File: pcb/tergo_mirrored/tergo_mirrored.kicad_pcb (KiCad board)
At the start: 2 copper layers, 140.5 x 100.6 mm, 63 parts, among them J3 MJ-4PP-9, SW1 SW_PUSH, SW10 SW_PUSH, SW11 SW_PUSH, SW12 SW_PUSH, SW13 SW_PUSH, SW14 SW_PUSH, SW15 SW_PUSH, SW16 SW_PUSH, SW17 SW_PUSH, SW18 SW_PUSH, SW19 SW_RESET, SW2 SW_PUSH, SW20 SW_PUSH, SW21 SW_PUSH, SW22 SW_PUSH, SW23 SW_PUSH, SW3 SW_PUSH, SW4 SW_PUSH, SW5 SW_PUSH, SW6 SW_PUSH, SW7 SW_PUSH, SW8 SW_PUSH, SW9 SW_PUSH, U1 Raspberry_Pie_Pico

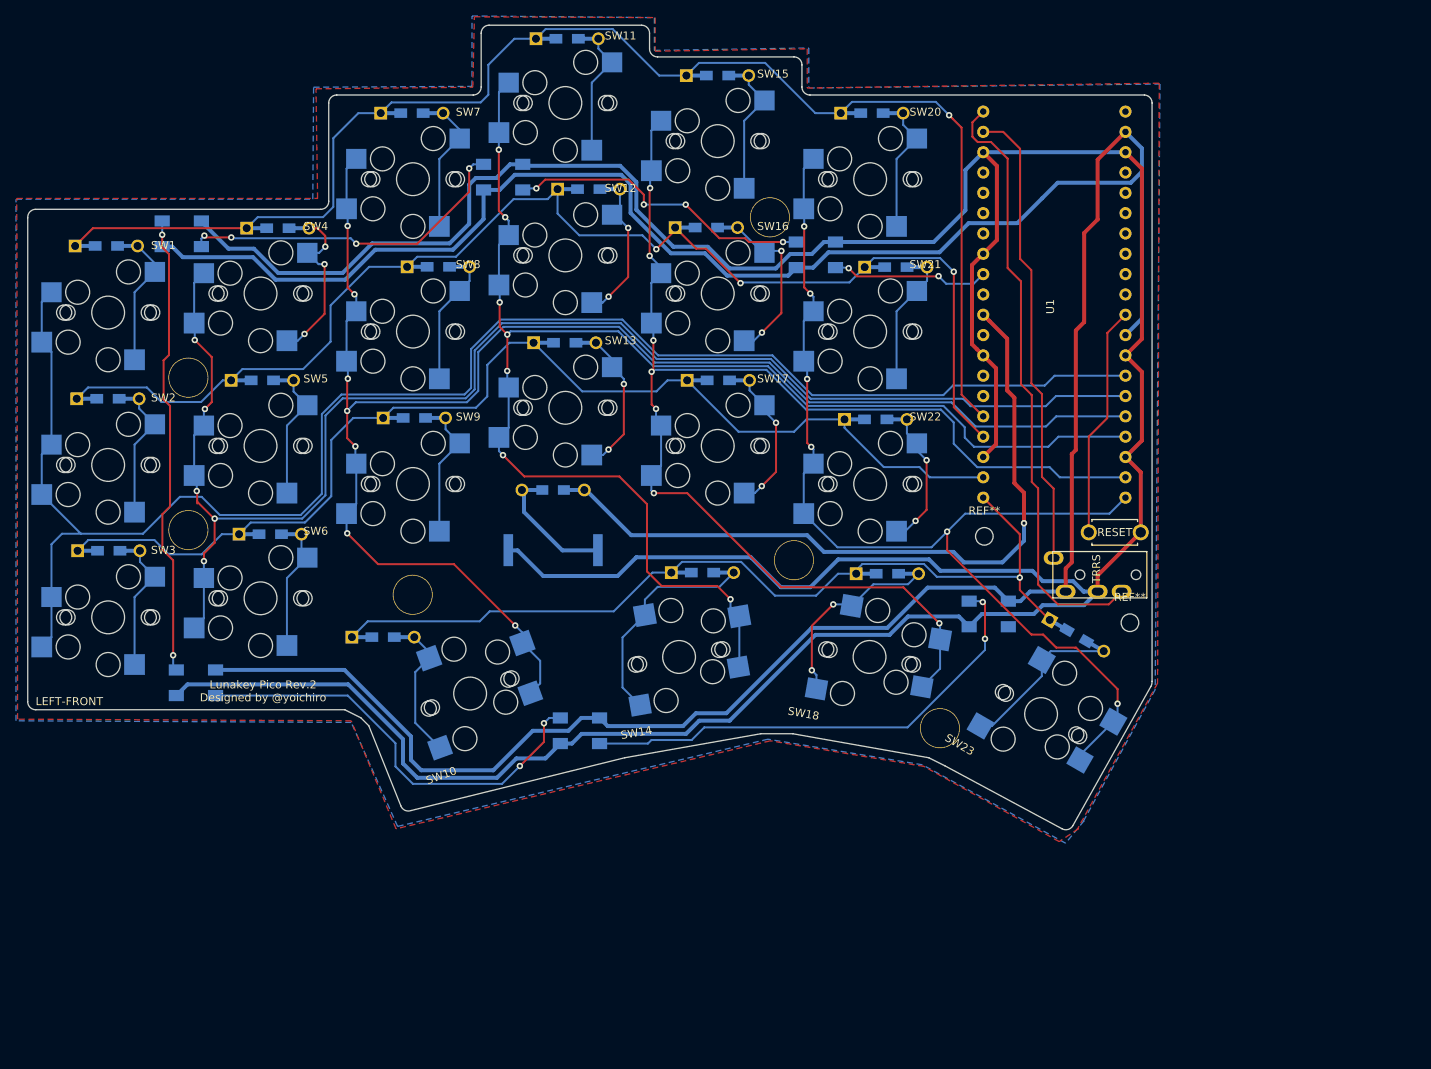
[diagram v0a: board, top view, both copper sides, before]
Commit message: wip
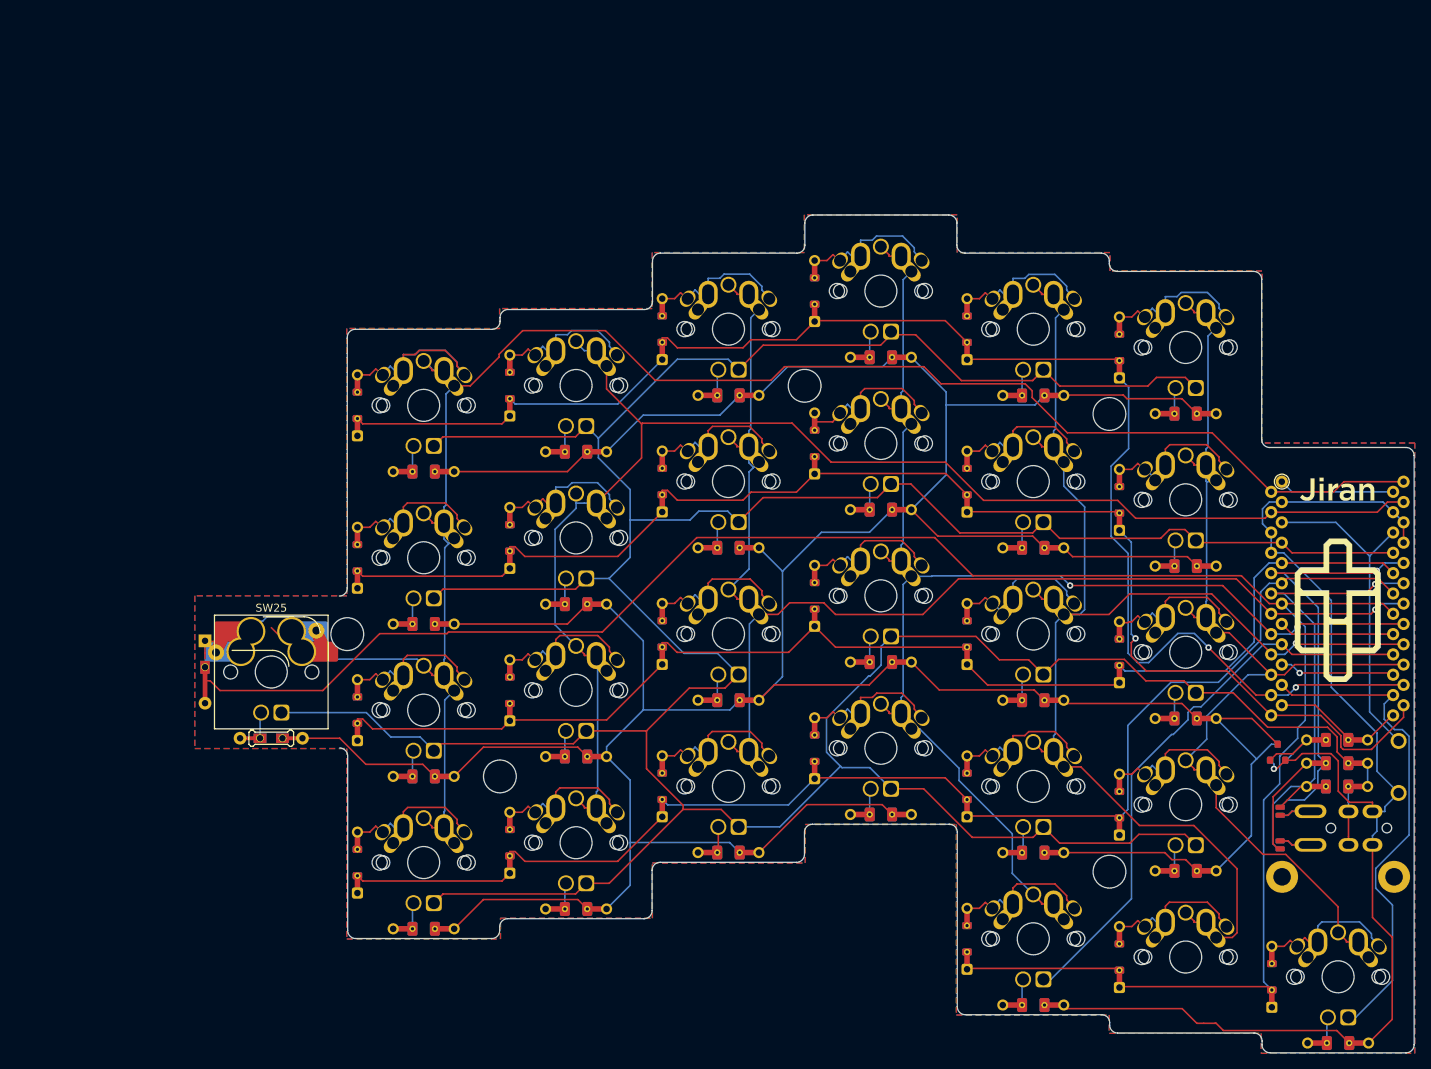
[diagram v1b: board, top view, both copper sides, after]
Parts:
- removed J3: MJ-4PP-9, kbd:MJ-4PP-9_1side
- removed LS1: PKLCS1212E4001-R1, _tergo_lib:PKLCS1212E4001-R1
- removed REF** (x2): COVER, MountingHole:MountingHole_2.2mm_M2
- removed Ref** (x6): Val**, kbd:HOLE
- added D23: 1N4148, Used_Footprints:Diode_Hybrid_SOD-123, F.Cu at (180.4, 180.7)
- added D24: 1N4148, Used_Footprints:Diode_Hybrid_SOD-123, F.Cu at (199.5, 183.0)
- added D25: 1N4148, _tergo_lib:Diode-Hybrid-2sided, F.Cu at (85.2, 166.4)
- added D26: 1N4148, Used_Footprints:Diode_Hybrid_SOD-123, F.Cu at (180.4, 199.7)
- added D27: 1N4148, Used_Footprints:Diode_Hybrid_SOD-123, F.Cu at (199.5, 202.0)
- added D28: 1N4148, Used_Footprints:Diode_Hybrid_SOD-123, F.Cu at (218.5, 204.5)
- added D29: LED_Small, Used_Footprints:LED, F.Cu at (112.5, 138.1)
- added D30: LED_Small, Used_Footprints:LED, F.Cu at (131.5, 135.6)
- added D31: LED_Small, Used_Footprints:LED, F.Cu at (150.6, 128.6)
- added D32: LED_Small, Used_Footprints:LED, F.Cu at (169.6, 123.8)
- added D33: LED_Small, Used_Footprints:LED, F.Cu at (188.7, 128.6)
- added D34: LED_Small, Used_Footprints:LED, F.Cu at (207.7, 130.9)
- added D35: LED_Small, Used_Footprints:LED, F.Cu at (112.5, 157.2)
- added D36: LED_Small, Used_Footprints:LED, F.Cu at (131.5, 154.7)
- added D37: LED_Small, Used_Footprints:LED, F.Cu at (150.6, 147.6)
- added D38: LED_Small, Used_Footprints:LED, F.Cu at (169.6, 142.9)
- added D39: LED_Small, Used_Footprints:LED, F.Cu at (188.7, 147.7)
- added D40: LED_Small, Used_Footprints:LED, F.Cu at (207.7, 149.9)
- added D41: LED_Small, Used_Footprints:LED, F.Cu at (112.5, 176.2)
- added D42: LED_Small, Used_Footprints:LED, F.Cu at (131.5, 173.7)
- added D43: LED_Small, Used_Footprints:LED, F.Cu at (150.6, 166.7)
- added D44: LED_Small, Used_Footprints:LED, F.Cu at (169.6, 161.9)
- added D50: LED_Small, Used_Footprints:LED, F.Cu at (169.6, 181.0)
- added D52: LED_Small, Used_Footprints:LED, F.Cu at (207.7, 188.0)
- added D53: LED_Small, Used_Footprints:LED, F.Cu at (93.4, 171.5)
- added D54: LED_Small, Used_Footprints:LED, F.Cu at (188.7, 204.8)
- added D56: LED_Small, Used_Footprints:LED, F.Cu at (226.8, 209.6)
- added G1: LOGO, Used_Footprints:Silk_Logo_Old, B.Cu at (226.7, 156.2)
- added G2: LOGO, Used_Footprints:Silk_Logo_Old, F.Cu at (226.8, 156.2)
- added H1: CaseHole, Used_Footprints:MountHole, F.Cu at (102.9, 161.6)
- added H2: CaseHole, Used_Footprints:MountHole, F.Cu at (122.0, 179.4)
- added H3: CaseHole, Used_Footprints:MountHole, F.Cu at (160.1, 130.6)
- added H6: CaseHole, Used_Footprints:MountHole, F.Cu at (198.2, 134.1)
- added H7: CaseHole, Used_Footprints:MountHole, F.Cu at (198.2, 191.3)
- added H8: CoverHole, Used_Footprints:CoverHole, F.Cu at (233.8, 192.0)
- added H9: CoverHole, Used_Footprints:CoverHole, F.Cu at (219.8, 192.0)
- added J1: TRRS, Used_Footprints:TRSS_DUAL_THT, F.Cu at (234.4, 185.9)
- added JP2: Jumper, 1kbd:jumper, B.Cu at (219.6, 183.8)
- added JP3: Jumper, 1kbd:jumper, F.Cu at (219.6, 183.8)
- added JP4: Jumper, 1kbd:jumper, F.Cu at (219.6, 188.0)
- added JP5: Jumper, 1kbd:jumper, B.Cu at (219.6, 188.0)
- added Q1: 2N7002, Used_Footprints:SOT-23, F.Cu at (219.2, 176.5)
- added R10: 330R, Used_Footprints:Resistor_Hybrid_1205, F.Cu at (169.6, 146.1)
- added R11: 330R, Used_Footprints:Resistor_Hybrid_1205, F.Cu at (188.7, 150.9)
- added R12: 330R, Used_Footprints:Resistor_Hybrid_1205, F.Cu at (207.7, 153.1)
- added R13: 330R, Used_Footprints:Resistor_Hybrid_1205, F.Cu at (112.5, 179.4)
- added R14: 330R, Used_Footprints:Resistor_Hybrid_1205, F.Cu at (131.5, 177.0)
- added R15: 330R, Used_Footprints:Resistor_Hybrid_1205, F.Cu at (150.6, 169.9)
- added R16: 330R, Used_Footprints:Resistor_Hybrid_1205, F.Cu at (169.6, 165.1)
- added R17: 330R, Used_Footprints:Resistor_Hybrid_1205, F.Cu at (188.7, 169.9)
- added R18: 330R, Used_Footprints:Resistor_Hybrid_1205, F.Cu at (207.7, 172.2)
- added R19: 330R, Used_Footprints:Resistor_Hybrid_1205, F.Cu at (112.5, 198.5)
- added R2: 330R, Used_Footprints:Resistor_Hybrid_1205, F.Cu at (131.5, 138.9)
- added R20: 330R, Used_Footprints:Resistor_Hybrid_1205, F.Cu at (131.5, 196.0)
- added R21: 330R, Used_Footprints:Resistor_Hybrid_1205, F.Cu at (150.6, 189.0)
- added R22: 330R, Used_Footprints:Resistor_Hybrid_1205, F.Cu at (169.6, 184.2)
- added R23: 330R, Used_Footprints:Resistor_Hybrid_1205, F.Cu at (188.7, 189.0)
- added R24: 330R, Used_Footprints:Resistor_Hybrid_1205, F.Cu at (207.7, 191.2)
- added R25: 330R, _tergo_lib:Resistor-Hybrid-2sided, F.Cu at (93.4, 174.7)
- added R26: 330R, Used_Footprints:Resistor_Hybrid_1205, F.Cu at (188.7, 208.0)
- added R28: 330R, Used_Footprints:Resistor_Hybrid_1205, F.Cu at (226.8, 212.8)
- added R29: 4.7k, Used_Footprints:Resistor_Hybrid_1205, F.Cu at (226.7, 177.8)
- added R3: 330R, Used_Footprints:Resistor_Hybrid_1205, F.Cu at (150.6, 131.8)
- added R30: 4.7k, Used_Footprints:Resistor_Hybrid_1205, F.Cu at (226.7, 180.7)
- added R31: 10k, Used_Footprints:Resistor_Hybrid_1205, F.Cu at (226.7, 174.9)
- added R4: 330R, Used_Footprints:Resistor_Hybrid_1205, F.Cu at (169.6, 127.0)
- added R5: 330R, Used_Footprints:Resistor_Hybrid_1205, F.Cu at (188.7, 131.8)
- added R6: 330R, Used_Footprints:Resistor_Hybrid_1205, F.Cu at (207.7, 134.1)
- added R7: 330R, Used_Footprints:Resistor_Hybrid_1205, F.Cu at (112.5, 160.4)
- added R8: 330R, Used_Footprints:Resistor_Hybrid_1205, F.Cu at (131.5, 157.9)
- added R9: 330R, Used_Footprints:Resistor_Hybrid_1205, F.Cu at (150.6, 150.9)
- added SW24: SW_Push, Used_Footprints:Switch_MxAlpsChoc_MillMax_1u, F.Cu at (207.7, 183.0)
- added SW25: SW_Push, _tergo_lib:SW_Hotswap_Kailh_MX_Plated_mirrored2_1.00u, F.Cu at (93.4, 166.4)
- added SW26: SW_Push, Used_Footprints:Switch_MxAlpsChoc_MillMax_1u, F.Cu at (188.7, 199.7)
- added SW27: SW_Push, Used_Footprints:Switch_MxAlpsChoc_MillMax_1u, F.Cu at (207.7, 202.0)
- added SW28: SW_Push, Used_Footprints:Switch_MxAlpsChoc_MillMax_1u, F.Cu at (226.8, 204.5)
- added SW29: SW_Push, Used_Footprints:Reset_Switch, F.Cu at (234.4, 178.3)
- D1, D10, D11, D12, D13, D14, D15, D16, D17, D18, D19, D2, D20, D21, D22, D3, D4, D5, D6, D7, D8, D9: value D -> 1N4148; footprint Keebio-Parts:Diode-Hybrid-Back -> Used_Footprints:Diode_Hybrid_SOD-123
- D45, D46, D47, D48, D49, D51: value WS2812B -> LED_Small; footprint _tergo_lib:Yoichiro-LED_WS2812B -> Used_Footprints:LED; moved to F.Cu
- R1: value 1k -> 330R; footprint _tergo_lib:Keebio-Resistor-Hybrid-Back -> Used_Footprints:Resistor_Hybrid_1205
- SW1, SW2: value SW_PUSH -> SW2; footprint _tergo_lib:CherryMX_Choco_Hotswap -> Used_Footprints:Switch_MxAlpsChoc_MillMax_1u
- SW10, SW11, SW12, SW13, SW14, SW15, SW16, SW17, SW18, SW20, SW21, SW22, SW23, SW3, SW4, SW5, SW6, SW7, SW8, SW9: value SW_PUSH -> SW_Push; footprint _tergo_lib:CherryMX_Choco_Hotswap -> Used_Footprints:Switch_MxAlpsChoc_MillMax_1u
- SW19: value SW_RESET -> SW_Push; footprint _tergo_lib:ResetSW -> Used_Footprints:Switch_MxAlpsChoc_MillMax_1u
- U1: value Raspberry_Pie_Pico -> ProMicro; footprint _tergo_lib:Raspberry_Pi_Pico -> Used_Footprints:ProMicro_TwoSide
- moved SW6 119.8 mm to (207.7, 125.8), turned to 180 degrees
- moved D19 113.6 mm to (104.2, 190.2), turned to 90 degrees
- moved D6 108.7 mm to (199.5, 125.8), turned to 90 degrees
- moved D45 104.7 mm to (188.7, 166.7), turned to 0 degrees
- moved SW5 97.7 mm to (188.7, 123.5), turned to 180 degrees
- moved SW19 95.7 mm to (112.5, 190.2)
- moved SW20 90.7 mm to (131.5, 187.7), turned to 180 degrees
- moved D47 89.0 mm to (112.5, 195.3)
- moved D5 88.3 mm to (180.4, 123.5), turned to 90 degrees
- moved D20 86.6 mm to (123.3, 187.7), turned to 90 degrees
- moved D49 86.0 mm to (150.6, 185.7)
- moved SW3 85.5 mm to (150.6, 123.5), turned to 180 degrees
- moved SW12 83.3 mm to (207.7, 144.9), turned to 180 degrees
- moved SW4 77.5 mm to (169.6, 118.8), turned to 180 degrees
- moved D12 76.9 mm to (199.5, 144.9), turned to 90 degrees
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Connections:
- D1 pad 1: row0-l -> /rowA
- D10 pad 1: row3-l -> /rowB
- D11 pad 1: row0-l -> /rowB
- D12 pad 1: row1-l -> /rowB
- D13 pad 1: row2-l -> /rowC
- D14 pad 1: row3-l -> /rowC
- D15 pad 1: row0-l -> /rowC
- D16 pad 1: row1-l -> /rowC
- D17 pad 1: row2-l -> /rowC
- D18 pad 1: row3-l -> /rowC
- D19 pad 1: row0-l -> /rowD
- D2 pad 1: row1-l -> /rowA
- D20 pad 1: row1-l -> /rowD
- D21 pad 1: row2-l -> /rowD
- D22 pad 1: row3-l -> /rowD
- D3 pad 1: row2-l -> /rowA
- D4 pad 1: row0-l -> /rowA
- D45 pad 1: VCC -> Net-(D45-Pad1)
- D45 pad 2: Net-(D45-Pad2) -> VCC
- D46 pad 1: VCC -> Net-(D46-Pad1)
- D46 pad 2: Net-(D46-Pad2) -> VCC
- D47 pad 1: VCC -> Net-(D47-Pad1)
- D47 pad 2: Net-(D45-Pad4) -> VCC
- D48 pad 1: VCC -> Net-(D48-Pad1)
- D48 pad 2: unconnected-(D48-Pad2) -> VCC
- D49 pad 1: VCC -> Net-(D49-Pad1)
- D49 pad 2: Net-(D47-Pad4) -> VCC
- D5 pad 1: row1-l -> /rowA
- D51 pad 1: VCC -> Net-(D51-Pad1)
- D51 pad 2: Net-(D49-Pad4) -> VCC
- D6 pad 1: row2-l -> /rowA
- D7 pad 1: row0-l -> /rowB
- D8 pad 1: row1-l -> /rowB
- D9 pad 1: row2-l -> /rowB
- R1 pad 2: audio-l -> /LEDOut
- SW1 pad 1: col0-l -> Net-(D2-Pad2)
- SW1 pad 2: Net-(D1-Pad2) -> /col1
- SW10 pad 1: col2-l -> Net-(D10-Pad2)
- SW10 pad 2: Net-(D10-Pad2) -> /col3
- SW11 pad 1: col3-l -> Net-(D11-Pad2)
- SW11 pad 2: Net-(D11-Pad2) -> /col4
- SW12 pad 1: col3-l -> Net-(D12-Pad2)
- SW12 pad 2: Net-(D12-Pad2) -> /col5
- SW13 pad 1: col3-l -> Net-(D13-Pad2)
- SW13 pad 2: Net-(D13-Pad2) -> /col0
- SW14 pad 1: col3-l -> Net-(D14-Pad2)
- SW14 pad 2: Net-(D14-Pad2) -> /col1
- SW15 pad 1: col4-l -> Net-(D15-Pad2)
- SW15 pad 2: Net-(D15-Pad2) -> /col2
- SW16 pad 1: col4-l -> Net-(D16-Pad2)
- SW16 pad 2: Net-(D16-Pad2) -> /col3
- SW17 pad 1: col4-l -> Net-(D17-Pad2)
- SW17 pad 2: Net-(D17-Pad2) -> /col4
- SW18 pad 1: col4-l -> Net-(D18-Pad2)
- SW18 pad 2: Net-(D18-Pad2) -> /col5
- SW19 pad 1: reset-l -> Net-(D19-Pad2)
- SW19 pad 2: GND -> /col0
- SW2 pad 1: col0-l -> Net-(D2-Pad2)
- SW2 pad 2: Net-(D2-Pad2) -> /col1
- SW20 pad 1: col5-l -> Net-(D20-Pad2)
- SW20 pad 2: Net-(D19-Pad2) -> /col1
- SW21 pad 1: col5-l -> Net-(D21-Pad2)
- SW21 pad 2: Net-(D20-Pad2) -> /col2
- SW22 pad 1: col5-l -> Net-(D22-Pad2)
- SW22 pad 2: Net-(D21-Pad2) -> /col3
- SW23 pad 1: col5-l -> Net-(D23-Pad2)
- SW23 pad 2: Net-(D22-Pad2) -> /col4
- SW3 pad 1: col0-l -> Net-(D3-Pad2)
- SW3 pad 2: Net-(D3-Pad2) -> /col2
- SW4 pad 1: col1-l -> Net-(D4-Pad2)
- SW4 pad 2: Net-(D4-Pad2) -> /col3
- SW5 pad 1: col1-l -> Net-(D5-Pad2)
- SW5 pad 2: Net-(D5-Pad2) -> /col4
- SW6 pad 1: col1-l -> Net-(D6-Pad2)
- SW6 pad 2: Net-(D6-Pad2) -> /col5
- SW7 pad 1: col2-l -> Net-(D7-Pad2)
- SW7 pad 2: Net-(D7-Pad2) -> /col0
- SW8 pad 1: col2-l -> Net-(D8-Pad2)
- SW8 pad 2: Net-(D8-Pad2) -> /col1
- SW9 pad 1: col2-l -> Net-(D9-Pad2)
- SW9 pad 2: Net-(D9-Pad2) -> /col2
- U1 pad 1: data-tx-l -> /col0
- U1 pad 10: unconnected-(U1-Pad10) -> /col5
- U1 pad 11: audio-l -> /rowA
- U1 pad 12: unconnected-(U1-Pad12) -> /rowB
- U1 pad 13: GND -> /LED
- U1 pad 14: unconnected-(U1-Pad14) -> /NUM
- U1 pad 15: unconnected-(U1-Pad15) -> /SCROLL
- U1 pad 16: row0-l -> /CAPS
- U1 pad 17: row1-l -> Net-(U1-Pad17)
- U1 pad 18: GND -> /rowE
- U1 pad 19: row2-l -> /rowD
- U1 pad 2: data-rx-l -> /col1
- U1 pad 20: row3-l -> /rowC
- U1 pad 21: col5-l -> VCC
- U1 pad 22: col4-l -> RST
- U1 pad 24: col3-l -> Net-(U1-Pad24)
- U1 pad 4: unconnected-(U1-Pad4) -> GND
- U1 pad 5: unconnected-(U1-Pad5) -> SDA
- U1 pad 6: unconnected-(U1-Pad6) -> SCL
- U1 pad 7: unconnected-(U1-Pad7) -> /col2
- U1 pad 8: GND -> /col3
- U1 pad 9: led-l -> /col4
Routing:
- net /LEDOut: track 0.00 -> 516.1 mm
- net GND: track 460.8 -> 163.8 mm, vias 0 -> 1
- net (no net): track 0.00 -> 267.5 mm
- net /rowE: track 0.00 -> 260.6 mm
- net col0-l: track 208.4 -> 0.00 mm
- net VCC: track 358.1 -> 563.7 mm
- net col2-l: track 195.6 -> 0.00 mm, vias 7 -> 0
- net /rowA: track 0.00 -> 191.9 mm, vias 0 -> 2
- net col1-l: track 189.3 -> 0.00 mm, vias 5 -> 0
- net col3-l: track 183.8 -> 0.00 mm, vias 7 -> 0
- net /col1: track 0.00 -> 183.6 mm
- net /rowB: track 0.00 -> 175.5 mm, vias 0 -> 1
- net row0-l: track 174.0 -> 0.00 mm, vias 1 -> 0
- net /col3: track 0.00 -> 173.3 mm, vias 0 -> 2
- net /rowD: track 0.00 -> 172.2 mm
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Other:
- board size 140.5 x 100.6 mm -> 134.3 x 104.7 mm
- board text removed: "LEFT-BACK"
- board text removed: "LEFT-FRONT"
- board text removed: "Lunakey Pico Rev.2 Designed by @yoichiro"
